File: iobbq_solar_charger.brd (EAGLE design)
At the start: 50 x 50 mm, 30 parts, among them X1 TE_RUUVULIITIN2, X2 TE_RUUVULIITIN2, X3 TE_RUUVULIITIN2, X4 TE_RUUVULIITIN2

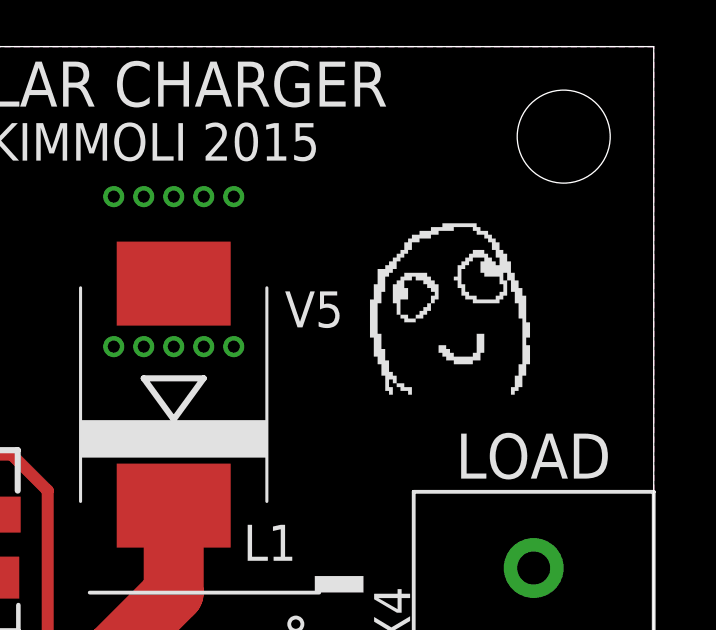
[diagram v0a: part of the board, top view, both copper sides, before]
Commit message: update values
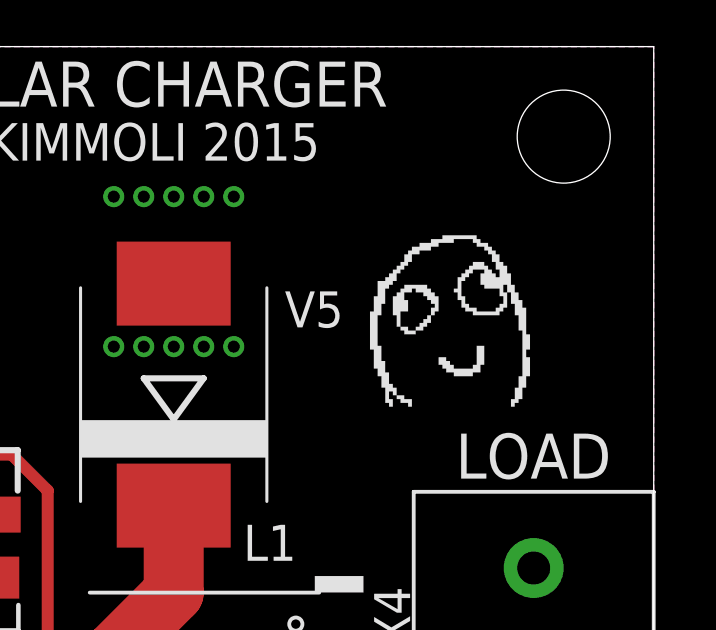
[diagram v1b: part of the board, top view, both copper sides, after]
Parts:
- removed U$1: (no value), dafug:DAFUG
- added U$2: DAFUG, dafug:DAFUG
- C2: value CAP0805 -> 4µ7
- C4: value CAP0805 -> 2µ2 50V
- H1: value (none) -> GRN
- H2: value (none) -> RED
- L1: value (none) -> WE-PD-7447779122
- R1, R2, R8: value RES0603 -> 100k
- R10, R9: value RES1206 -> 2k15
- R11: value RES1206 -> 0.1R 1206
- R3: value RES0603 -> NCP18XH103
- R4: value RES0603 -> 910R
- R5: value RES0603 -> 174k
- R6: value RES0603 -> 1M
- R7: value RES0603 -> 309k
- V1, V5: value (none) -> MBRS340
- V4: value BZX84CSMD -> BZX84C 6V2
- X1, X2, X3, X4: value TE_RUUVULIITIN2 -> TE 282837-2
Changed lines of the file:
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@@
 <attribute name="VALUE" x="25.3472" y="34.412" size="2.0828" layer="27" ratio="10" rot="SR90"/>
 </element>
-<element name="C2" library="OMAT_IC" package="C0805" value="CAP0805" x="21" y="21" smashed="yes" rot="R270">
+<element name="C2" library="OMAT_IC" package="C0805" value="4µ7" x="21" y="21" smashed="yes" rot="R270">
 <attribute name="NAME" x="22.27" y="22.27" size="1.2" layer="25" font="vector" rot="R270"/>
 <attribute name="VALUE" x="18.46" y="22.27" size="0.8128" layer="27" rot="R270"/>
@@
 <attribute name="VALUE" x="21.6528" y="13.588" size="2.0828" layer="27" ratio="10" rot="SR270"/>
 </element>
-<element name="C4" library="OMAT_IC" package="C0805" value="CAP0805" x="35.8" y="18.6" smashed="yes">
+<element name="C4" library="OMAT_IC" package="C0805" value="2µ2 50V" x="35.8" y="18.6" smashed="yes">
 <attribute name="NAME" x="34.73" y="16.27" size="1.2" layer="25" font="vector"/>
 <attribute name="VALUE" x="34.53" y="16.06" size="0.8128" layer="27"/>
 </element>
-<element name="V4" library="diode" package="TO236" value="BZX84CSMD" x="27.4" y="35.4" smashed="yes">
+<element name="V4" library="diode" package="TO236" value="BZX84C 6V2" x="27.4" y="35.4" smashed="yes">
 <attribute name="NAME" x="26.003" y="37.194" size="1.2" layer="25" font="vector"/>
 <attribute name="VALUE" x="25.876" y="32.336" size="1.27" layer="27"/>
 </element>
-<element name="V5" library="diode" package="SMC" value="" x="34" y="38.4" smashed="yes" rot="R90">
+<element name="V5" library="diode" package="SMC" value="MBRS340" x="34" y="38.4" smashed="yes" rot="R90">
 <attribute name="NAME" x="39.659" y="41.841" size="1.2" layer="25" font="vector" rot="R180"/>
 <attribute name="VALUE" x="38.629" y="34.941" size="1.27" layer="27" rot="R90"/>
 </element>
-<element name="V1" library="diode" package="SMC" value="" x="4" y="37" smashed="yes" rot="R270">
+<element name="V1" library="diode" package="SMC" value="MBRS340" x="4" y="37" smashed="yes" rot="R270">
 <attribute name="NAME" x="8.659" y="33.041" size="1.2" layer="25" font="vector" rot="R180"/>
 <attribute name="VALUE" x="-0.629" y="40.459" size="1.27" layer="27" rot="R270"/>
 </element>
-<element name="L1" library="WE-PD" package="WE-PD_7332/7345_PLASTIC_BASE" value="" x="35" y="28" smashed="yes" rot="R270">
+<element name="L1" library="WE-PD" package="WE-PD_7332/7345_PLASTIC_BASE" value="WE-PD-7447779122" x="35" y="28" smashed="yes" rot="R270">
 <attribute name="PACKAGE" value="7345" x="35" y="28" size="1.778" layer="27" rot="R270" display="off"/>
 <attribute name="OC_NEWARK" value="08P2860" x="35" y="28" size="1.778" layer="27" rot="R270" display="off"/>
@@
 <attribute name="VALUE" x="30.76" y="21.55" size="1.27" layer="27"/>
 </element>
-<element name="H1" library="OMAT_IC" package="LED3MM" value="" x="12.54" y="12" smashed="yes">
+<element name="H1" library="OMAT_IC" package="LED3MM" value="GRN" x="12.54" y="12" smashed="yes">
 <attribute name="NAME" x="11.645" y="8.381" size="1.2" layer="25" font="vector" ratio="10"/>
 <attribute name="VALUE" x="14.445" y="10.349" size="1.27" layer="27" ratio="10"/>
 </element>
-<element name="H2" library="OMAT_IC" package="LED3MM" value="" x="17.62" y="12" smashed="yes">
+<element name="H2" library="OMAT_IC" package="LED3MM" value="RED" x="17.62" y="12" smashed="yes">
 <attribute name="NAME" x="16.725" y="8.381" size="1.2" layer="25" font="vector" ratio="10"/>
 <attribute name="VALUE" x="19.525" y="10.349" size="1.27" layer="27" ratio="10"/>
@@
 <attribute name="VALUE" x="21.5456" y="21.68" size="0.9" layer="27" font="vector" ratio="10" rot="SR0"/>
 </element>
-<element name="R10" library="OMAT_IC" package="R1206" value="RES1206" x="21.25" y="12.02" smashed="yes" rot="R270">
+<element name="R10" library="OMAT_IC" package="R1206" value="2k15" x="21.25" y="12.02" smashed="yes" rot="R270">
 <attribute name="NAME" x="22.52" y="13.89" size="1.2" layer="25" font="vector" rot="R270"/>
 <attribute name="VALUE" x="18.71" y="13.29" size="1.27" layer="27" rot="R270"/>
 </element>
-<element name="R9" library="OMAT_IC" package="R1206" value="RES1206" x="8.65" y="11.98" smashed="yes" rot="R270">
+<element name="R9" library="OMAT_IC" package="R1206" value="2k15" x="8.65" y="11.98" smashed="yes" rot="R270">
 <attribute name="NAME" x="6.12" y="13.25" size="1.2" layer="25" font="vector" rot="R270"/>
 <attribute name="VALUE" x="6.11" y="13.25" size="1.27" layer="27" rot="R270"/>
 </element>
-<element name="R1" library="OMAT_IC" package="R0603" value="RES0603" x="15" y="25" smashed="yes">
+<element name="R1" library="OMAT_IC" package="R0603" value="100k" x="15" y="25" smashed="yes">
 <attribute name="NAME" x="16.565" y="24.435" size="1.2" layer="25" font="vector"/>
 <attribute name="VALUE" x="14.365" y="23.095" size="0.8128" layer="27"/>
 </element>
-<element name="R2" library="OMAT_IC" package="R0603" value="RES0603" x="15" y="27" smashed="yes">
+<element name="R2" library="OMAT_IC" package="R0603" value="100k" x="15" y="27" smashed="yes">
 <attribute name="NAME" x="16.565" y="26.435" size="1.2" layer="25" font="vector"/>
 <attribute name="VALUE" x="14.365" y="25.095" size="0.8128" layer="27"/>
 </element>
-<element name="R11" library="OMAT_IC" package="R1206" value="RES1206" x="35" y="22" smashed="yes" rot="R180">
+<element name="R11" library="OMAT_IC" package="R1206" value="0.1R 1206" x="35" y="22" smashed="yes" rot="R180">
 <attribute name="NAME" x="35.87" y="20.93" size="1.2" layer="25" font="vector" rot="R180"/>
 <attribute name="VALUE" x="36.27" y="24.54" size="1.27" layer="27" rot="R180"/>
 </element>
-<element name="R4" library="OMAT_IC" package="R0603" value="RES0603" x="42.2" y="8" smashed="yes" rot="R180">
+<element name="R4" library="OMAT_IC" package="R0603" value="910R" x="42.2" y="8" smashed="yes" rot="R180">
 <attribute name="NAME" x="43.435" y="6.965" size="1.2" layer="25" font="vector" rot="R180"/>
 <attribute name="VALUE" x="42.835" y="9.905" size="0.8128" layer="27" rot="R180"/>
 </element>
-<element name="R3" library="OMAT_IC" package="R0603" value="RES0603" x="47.4" y="8" smashed="yes" rot="R180">
+<element name="R3" library="OMAT_IC" package="R0603" value="NCP18XH103" x="47.4" y="8" smashed="yes" rot="R180">
 <attribute name="NAME" x="48.635" y="6.965" size="1.2" layer="25" font="vector" rot="R180"/>
 <attribute name="VALUE" x="48.035" y="9.905" size="0.8128" layer="27" rot="R180"/>
 </element>
-<element name="R7" library="OMAT_IC" package="R0603" value="RES0603" x="30" y="19" smashed="yes">
+<element name="R7" library="OMAT_IC" package="R0603" value="309k" x="30" y="19" smashed="yes">
 <attribute name="NAME" x="28.965" y="19.835" size="1.2" layer="25" font="vector"/>
 <attribute name="VALUE" x="29.365" y="17.095" size="0.8128" layer="27"/>
 </element>
-<element name="R6" library="OMAT_IC" package="R0603" value="RES0603" x="16" y="21" smashed="yes" rot="R270">
+<element name="R6" library="OMAT_IC" package="R0603" value="1M" x="16" y="21" smashed="yes" rot="R270">
 <attribute name="NAME" x="13.835" y="22.035" size="1.2" layer="25" font="vector" rot="R270"/>
 <attribute name="VALUE" x="14.095" y="21.635" size="0.8128" layer="27" rot="R270"/>
 </element>
-<element name="R5" library="OMAT_IC" package="R0603" value="RES0603" x="27" y="21" smashed="yes">
+<element name="R5" library="OMAT_IC" package="R0603" value="174k" x="27" y="21" smashed="yes">
 <attribute name="NAME" x="26.365" y="21.835" size="1.2" layer="25" font="vector"/>
 <attribute name="VALUE" x="26.365" y="19.095" size="0.8128" layer="27"/>
 </element>
-<element name="R8" library="OMAT_IC" package="R0603" value="RES0603" x="27" y="19" smashed="yes">
+<element name="R8" library="OMAT_IC" package="R0603" value="100k" x="27" y="19" smashed="yes">
 <attribute name="NAME" x="26.165" y="17.035" size="1.2" layer="25" font="vector"/>
 <attribute name="VALUE" x="26.365" y="17.095" size="0.8128" layer="27"/>
@@
 <attribute name="VALUE" x="21.175" y="16.495" size="1.27" layer="27" rot="R90"/>
 </element>
-<element name="X2" library="OMAT_IC" package="TE_RUUVILIITIN2" value="TE_RUUVULIITIN2" x="12.54" y="4" smashed="yes">
+<element name="X2" library="OMAT_IC" package="TE_RUUVILIITIN2" value="TE 282837-2" x="12.54" y="4" smashed="yes">
 <attribute name="NAME" x="14" y="8.48" size="1.2" layer="25" font="vector"/>
 </element>
-<element name="X1" library="OMAT_IC" package="TE_RUUVILIITIN2" value="TE_RUUVULIITIN2" x="4" y="27.54" smashed="yes" rot="R270">
+<element name="X1" library="OMAT_IC" package="TE_RUUVILIITIN2" value="TE 282837-2" x="4" y="27.54" smashed="yes" rot="R270">
 <attribute name="NAME" x="8.32" y="24.28" size="1.2" layer="25" font="vector"/>
 </element>
-<element name="X4" library="OMAT_IC" package="TE_RUUVILIITIN2" value="TE_RUUVULIITIN2" x="46" y="27.54" smashed="yes" rot="R90">
+<element name="X4" library="OMAT_IC" package="TE_RUUVILIITIN2" value="TE 282837-2" x="46" y="27.54" smashed="yes" rot="R90">
 <attribute name="NAME" x="40.68" y="32" size="1.2" layer="25" font="vector" rot="R270"/>
 </element>
-<element name="X3" library="OMAT_IC" package="TE_RUUVILIITIN2" value="TE_RUUVULIITIN2" x="46" y="17.38" smashed="yes" rot="R90">
+<element name="X3" library="OMAT_IC" package="TE_RUUVILIITIN2" value="TE 282837-2" x="46" y="17.38" smashed="yes" rot="R90">
 <attribute name="NAME" x="40.68" y="20.96" size="1.2" layer="25" font="vector" rot="R270"/>
 </element>
-<element name="U$1" library="dafug" package="DAFUG" value="" x="43.4" y="41"/>
+<element name="U$2" library="dafug" package="DAFUG" value="DAFUG" x="43.4" y="40.6"/>
 </elements>
 <signals>
